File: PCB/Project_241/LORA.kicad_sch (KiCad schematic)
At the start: 1 part, among them U4 RA02

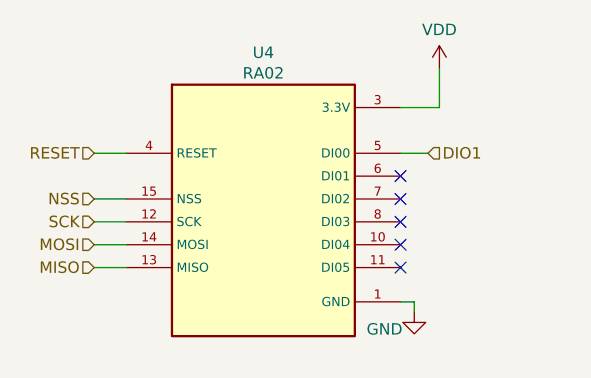
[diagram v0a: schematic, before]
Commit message: update gerber
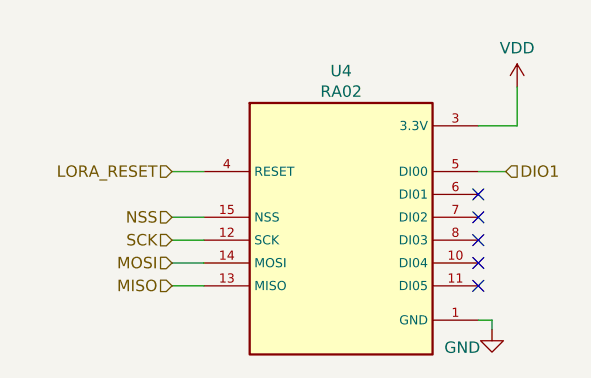
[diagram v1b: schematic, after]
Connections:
- net RESET renamed LORA_RESET
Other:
- moved on the sheet: U4
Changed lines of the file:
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@@
 	(paper "A4")
 	(no_connect
-		(at 154.686 99.568)
-	)
-	(no_connect
-		(at 154.686 89.408)
-	)
-	(no_connect
-		(at 154.686 94.488)
-	)
-	(no_connect
-		(at 154.686 91.948)
-	)
-	(no_connect
-		(at 154.686 97.028)
-	)
-	(wire
-		(pts
-			(xy 159.004 81.788) (xy 154.686 81.788)
-		)
-		(stroke
-			(width 0)
-			(type default)
-		)
-	)
-	(wire
-		(pts
-			(xy 120.65 91.948) (xy 124.206 91.948)
-		)
-		(stroke
-			(width 0)
-			(type default)
-		)
-	)
-	(wire
-		(pts
-			(xy 120.65 97.028) (xy 124.206 97.028)
-		)
-		(stroke
-			(width 0)
-			(type default)
-		)
-	)
-	(wire
-		(pts
-			(xy 120.65 94.488) (xy 124.206 94.488)
-		)
-		(stroke
-			(width 0)
-			(type default)
-		)
-	)
-	(wire
-		(pts
-			(xy 157.734 86.868) (xy 154.686 86.868)
-		)
-		(stroke
-			(width 0)
-			(type default)
-		)
-	)
-	(wire
-		(pts
-			(xy 120.65 86.868) (xy 124.206 86.868)
-		)
-		(stroke
-			(width 0)
-			(type default)
-		)
-	)
-	(wire
-		(pts
-			(xy 156.21 104.394) (xy 156.21 103.378)
-		)
-		(stroke
-			(width 0)
-			(type default)
-		)
-	)
-	(wire
-		(pts
-			(xy 159.004 77.47) (xy 159.004 81.788)
-		)
-		(stroke
-			(width 0)
-			(type default)
-		)
-	)
-	(wire
-		(pts
-			(xy 120.65 99.568) (xy 124.206 99.568)
-		)
-		(stroke
-			(width 0)
-			(type default)
-		)
-	)
-	(wire
-		(pts
-			(xy 156.21 103.378) (xy 154.686 103.378)
+		(at 163.322 101.6)
+	)
+	(no_connect
+		(at 163.322 91.44)
+	)
+	(no_connect
+		(at 163.322 96.52)
+	)
+	(no_connect
+		(at 163.322 93.98)
+	)
+	(no_connect
+		(at 163.322 99.06)
+	)
+	(wire
+		(pts
+			(xy 167.64 83.82) (xy 163.322 83.82)
+		)
+		(stroke
+			(width 0)
+			(type default)
+		)
+	)
+	(wire
+		(pts
+			(xy 129.286 93.98) (xy 132.842 93.98)
+		)
+		(stroke
+			(width 0)
+			(type default)
+		)
+	)
+	(wire
+		(pts
+			(xy 129.286 99.06) (xy 132.842 99.06)
+		)
+		(stroke
+			(width 0)
+			(type default)
+		)
+	)
+	(wire
+		(pts
+			(xy 129.286 96.52) (xy 132.842 96.52)
+		)
+		(stroke
+			(width 0)
+			(type default)
+		)
+	)
+	(wire
+		(pts
+			(xy 166.37 88.9) (xy 163.322 88.9)
+		)
+		(stroke
+			(width 0)
+			(type default)
+		)
+	)
+	(wire
+		(pts
+			(xy 129.286 88.9) (xy 132.842 88.9)
+		)
+		(stroke
+			(width 0)
+			(type default)
+		)
+	)
+	(wire
+		(pts
+			(xy 164.846 106.426) (xy 164.846 105.41)
+		)
+		(stroke
+			(width 0)
+			(type default)
+		)
+	)
+	(wire
+		(pts
+			(xy 167.64 79.502) (xy 167.64 83.82)
+		)
+		(stroke
+			(width 0)
+			(type default)
+		)
+	)
+	(wire
+		(pts
+			(xy 129.286 101.6) (xy 132.842 101.6)
+		)
+		(stroke
+			(width 0)
+			(type default)
+		)
+	)
+	(wire
+		(pts
+			(xy 164.846 105.41) (xy 163.322 105.41)
 		)
 		(stroke
@@
 	(hierarchical_label "SCK"
 		(shape input)
-		(at 120.65 94.488 180)
+		(at 129.286 96.52 180)
 		(fields_autoplaced yes)
 		(effects
@@
 	(hierarchical_label "DIO1"
 		(shape input)
-		(at 157.734 86.868 0)
+		(at 166.37 88.9 0)
 		(fields_autoplaced yes)
 		(effects
@@
 		)
 	)
-	(hierarchical_label "RESET"
-		(shape input)
-		(at 120.65 86.868 180)
+	(hierarchical_label "LORA_RESET"
+		(shape input)
+		(at 129.286 88.9 180)
 		(fields_autoplaced yes)
 		(effects
@@
 	(hierarchical_label "NSS"
 		(shape input)
-		(at 120.65 91.948 180)
+		(at 129.286 93.98 180)
 		(fields_autoplaced yes)
 		(effects
@@
 	(hierarchical_label "MISO"
 		(shape input)
-		(at 120.65 99.568 180)
+		(at 129.286 101.6 180)
 		(fields_autoplaced yes)
 		(effects
@@
 	(hierarchical_label "MOSI"
 		(shape input)
-		(at 120.65 97.028 180)
+		(at 129.286 99.06 180)
 		(fields_autoplaced yes)
 		(effects
@@
 	(symbol
 		(lib_id "power:GND")
-		(at 156.21 104.394 0)
+		(at 164.846 106.426 0)
 		(unit 1)
 		(exclude_from_sim no)
@@
 		(dnp no)
 		(property "Reference" "#PWR039"
-			(at 156.21 110.744 0)
+			(at 164.846 112.776 0)
 			(effects
 				(font
@@
 		)
 		(property "Value" "GND"
-			(at 152.908 106.426 0)
+			(at 161.544 108.458 0)
 			(effects
 				(font
@@
 		)
 		(property "Footprint" ""
-			(at 156.21 104.394 0)
+			(at 164.846 106.426 0)
 			(effects
 				(font
@@
 		)
 		(property "Datasheet" ""
-			(at 156.21 104.394 0)
+			(at 164.846 106.426 0)
 			(effects
 				(font
@@
 		)
 		(property "Description" "Power symbol creates a global label with name \"GND\" , ground"
-			(at 156.21 104.394 0)
+			(at 164.846 106.426 0)
 			(effects
 				(font
@@
 	(symbol
 		(lib_id "power:VDD")
-		(at 159.004 77.47 0)
+		(at 167.64 79.502 0)
 		(unit 1)
 		(exclude_from_sim no)
@@
 		(fields_autoplaced yes)
 		(property "Reference" "#PWR038"
-			(at 159.004 81.28 0)
+			(at 167.64 83.312 0)
 			(effects
 				(font
@@
 		)
 		(property "Value" "VDD"
-			(at 159.004 73.152 0)
+			(at 167.64 75.184 0)
 			(effects
 				(font
@@
 		)
 		(property "Footprint" ""
-			(at 159.004 77.47 0)
+			(at 167.64 79.502 0)
 			(effects
 				(font
@@
 		)
 		(property "Datasheet" ""
-			(at 159.004 77.47 0)
+			(at 167.64 79.502 0)
 			(effects
 				(font
@@
 		)
 		(property "Description" "Power symbol creates a global label with name \"VDD\""
-			(at 159.004 77.47 0)
+			(at 167.64 79.502 0)
 			(effects
 				(font
@@
 	(symbol
 		(lib_id "project241_sym:Lora_RA_02")
-		(at 139.446 93.218 0)
+		(at 148.082 95.25 0)
 		(unit 1)
 		(exclude_from_sim no)
@@
 		(dnp no)
 		(property "Reference" "U4"
-			(at 139.446 75.692 0)
+			(at 148.082 77.724 0)
 			(effects
 				(font
@@
 		)
 		(property "Value" "RA02"
-			(at 139.446 77.978 0)
+			(at 148.082 80.01 0)
 			(effects
 				(font
@@
 		)
 		(property "Footprint" "project241_footprint:RA-02"
-			(at 138.176 110.998 0)
+			(at 146.812 113.03 0)
 			(effects
 				(font
@@
 		)
 		(property "Datasheet" ""
-			(at 139.446 91.948 0)
+			(at 148.082 93.98 0)
 			(effects
 				(font
@@
 		)
 		(property "Description" ""
-			(at 139.446 91.948 0)
-			(effects
-				(font
+			(at 148.082 93.98 0)
+			(effects
+				(font
